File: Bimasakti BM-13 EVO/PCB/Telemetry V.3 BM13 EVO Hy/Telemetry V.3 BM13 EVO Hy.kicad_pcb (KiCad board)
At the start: 2 copper layers, 23 parts, among them J1 MSD-4-A, J2 CON INT/32, J3 CON Power, U1 ESP32-DEVKIT-V1, U2 74LVC125APW_118, U3 DS3231SN_

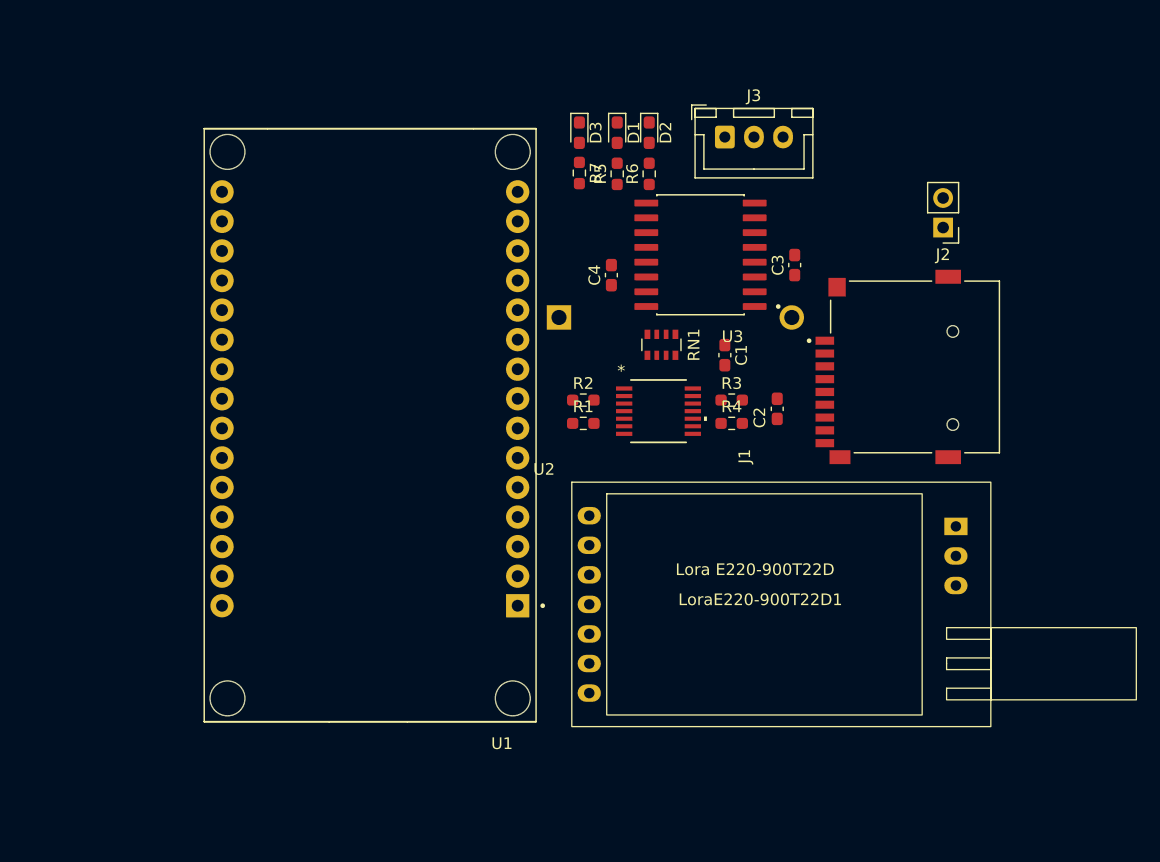
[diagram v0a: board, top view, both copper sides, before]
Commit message: Arjun Update Finish Telemetry
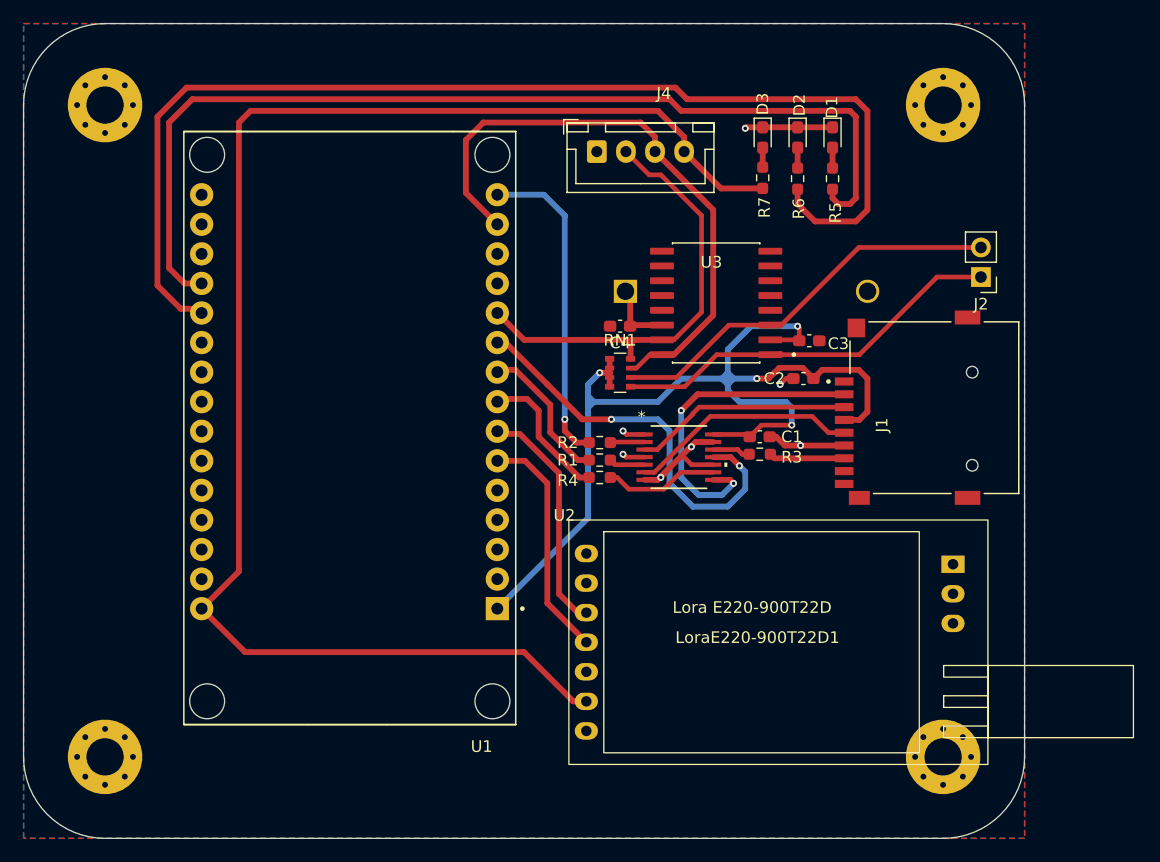
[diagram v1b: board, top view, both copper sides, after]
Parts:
- removed J3: CON Power, Connector_JST:JST_XH_B3B-XH-A_1x03_P2.50mm_Vertical
- added J4: Conn_01x04_Socket, Connector_JST:JST_XH_B4B-XH-A_1x04_P2.50mm_Vertical, F.Cu at (96.8, 56.0)
- added REF**: MountingHole_3.2mm_M3_Pad_Via, MountingHole:MountingHole_3.2mm_M3_Pad_Via, F.Cu at (54.5, 52.0)
- added REF**: MountingHole_3.2mm_M3_Pad_Via, MountingHole:MountingHole_3.2mm_M3_Pad_Via, F.Cu at (126.5, 108.0)
- added REF**: MountingHole_3.2mm_M3_Pad_Via, MountingHole:MountingHole_3.2mm_M3_Pad_Via, F.Cu at (126.5, 52.0)
- added REF**: MountingHole_3.2mm_M3_Pad_Via, MountingHole:MountingHole_3.2mm_M3_Pad_Via, F.Cu at (54.5, 108.0)
- BT1: footprint Battery:BatteryHolder_ComfortableElectronic_CH273-2450_1x2450 -> Battery:BatteryHolder_MYOUNG_BS-07-A1BJ001_CR2032
- D1: value LED -> RTC
- D2: value LED -> SDCard
- D3: value LED -> 5V
- moved D1 18.5 mm to (117.0, 54.8)
- moved R5 18.5 mm to (117.0, 58.3)
- moved D3 15.8 mm to (111.0, 54.8)
- moved R7 15.8 mm to (111.0, 58.2)
- moved D2 12.8 mm to (114.0, 54.8)
- moved R6 12.8 mm to (114.0, 58.3)
- moved R4 12.3 mm to (97.0, 84.0), turned to 180 degrees
- moved C1 7.63 mm to (110.8, 80.5), turned to 180 degrees
- moved C3 6.62 mm to (115.0, 72.2), turned to 180 degrees
- moved BT1 6.14 mm to (99.2, 68.0)
- moved J2 5.35 mm to (129.8, 66.8)
- moved R3 5.24 mm to (110.8, 82.0)
- moved C4 4.45 mm to (98.8, 71.0), turned to 180 degrees
- moved U3 4.35 mm to (107.0, 69.0)
- moved U2 4.32 mm to (103.8, 82.2)
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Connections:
- RN1 pad 5: /SCL -> /32KHz
- RN1 pad 6: /SDA -> /SQW
- RN1 pad 7: /32KHz -> /SCL
- RN1 pad 8: /SQW -> /SDA
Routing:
- net +5V: track 0.00 -> 128.3 mm
- net /LED1: track 0.00 -> 98.9 mm
- net +3.3V: track 0.00 -> 91.8 mm, vias 0 -> 4
- net /LED2: track 0.00 -> 86.5 mm
- net /SCL: track 0.00 -> 52.1 mm
- net /SDA: track 0.00 -> 40.3 mm
- net /MISO: track 0.00 -> 35.2 mm, vias 0 -> 2
- net /SQW: track 0.00 -> 34.7 mm
- net /32KHz: track 0.00 -> 34.1 mm
- net GND: track 0.00 -> 30.7 mm, vias 0 -> 7
- net /CS_LLS: track 0.00 -> 27.7 mm, vias 0 -> 2
- net /MOSI: track 0.00 -> 27.5 mm, vias 0 -> 1
- net /RX: track 0.00 -> 20.2 mm
- net /TX: track 0.00 -> 20.1 mm
- net /SCK_LLS: track 0.00 -> 19.7 mm
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- added copper zone on B.Cu, net GND
- added copper zone on F.Cu, net GND
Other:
- board outline added: 86 x 70 mm
- board text added: "32"
- board text added: "5V"
- board text added: "GND"
- board text added: "Indicator"
- board text added: "RTC"
- board text added: "SCL"
- board text added: "SD CARD"
- board text added: "SDA"
- board text added: "SQW"
